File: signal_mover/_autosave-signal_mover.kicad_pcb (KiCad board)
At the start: 2 copper layers, 20.8 x 14.7 mm, 4 parts, among them P1 CONN_01X03

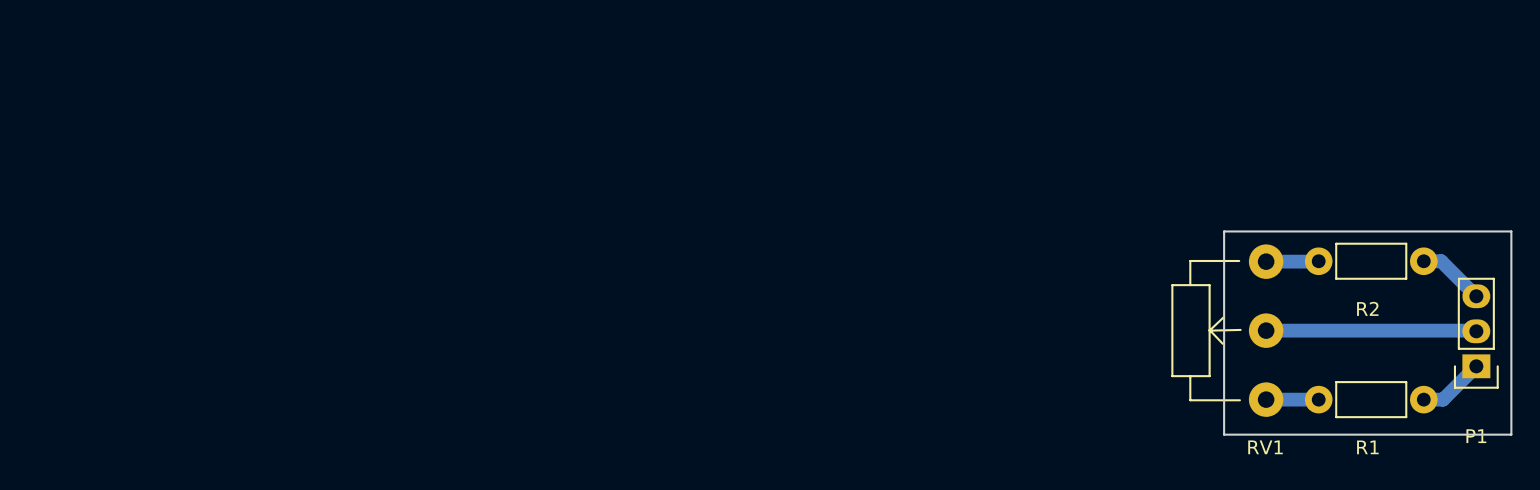
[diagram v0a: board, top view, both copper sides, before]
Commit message: updated signal mover
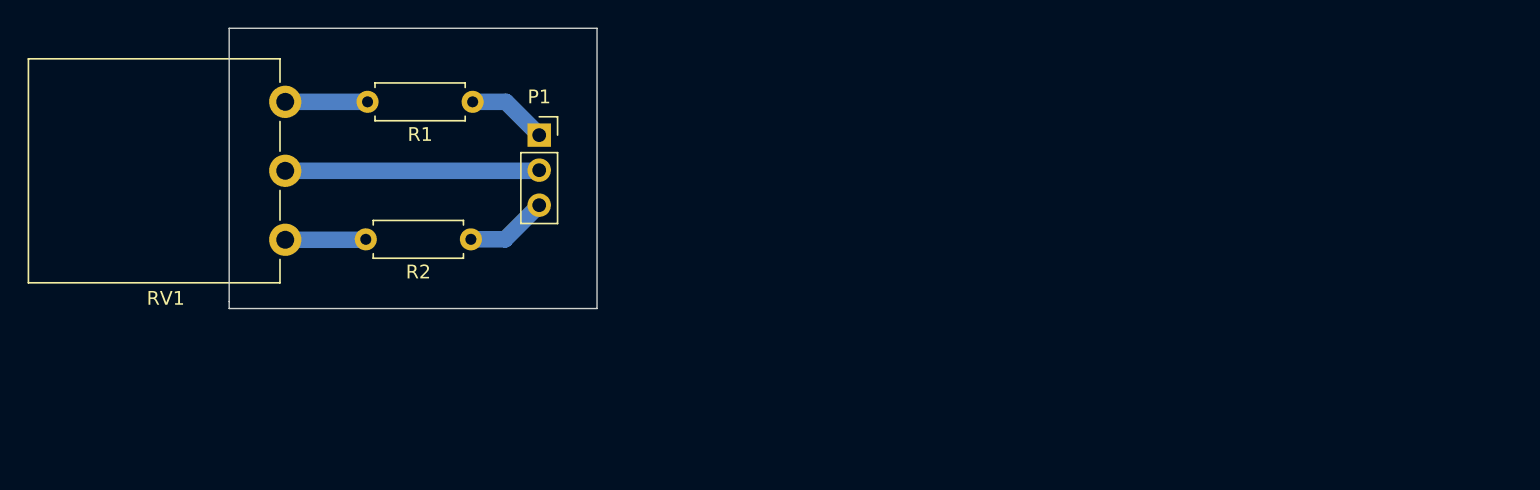
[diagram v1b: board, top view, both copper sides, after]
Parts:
- P1: footprint Pin_Headers:Pin_Header_Straight_1x03 -> Connector_PinSocket_2.54mm:PinSocket_1x03_P2.54mm_Vertical
- R1, R2: footprint Resistors_ThroughHole:Resistor_Horizontal_RM7mm -> Resistor_THT:R_Axial_DIN0207_L6.3mm_D2.5mm_P7.62mm_Horizontal
- RV1: footprint Potentiometers:Potentiometer_WirePads_largePads -> Potentiometer_THT:Potentiometer_Piher_PC-16_Single_Vertical
- moved RV1 74.3 mm to (67.6, 89.2)
- moved R1 72.3 mm to (81.2, 89.2)
- moved P1 70.0 mm to (86.0, 91.6), turned to 0 degrees
- moved R2 69.1 mm to (81.0, 99.1)
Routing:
- net Net-(P1-Pad2): track 15.3 -> 17.9 mm
- net Net-(R1-Pad2): track 3.81 -> 5.46 mm
- net Net-(R2-Pad2): track 3.82 -> 5.35 mm
- net Net-(P1-Pad3): track 4.86 -> 5.98 mm
- net Net-(P1-Pad1): track 4.81 -> 5.83 mm
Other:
- board size 20.8 x 14.7 mm -> 26.7 x 20.3 mm
- net class Default: clearance 0.3 -> 0.2; trace_width 1 -> 1.2; via_dia 0.6 -> 0.8
- rule pad_to_mask_clearance: 0.2 -> 0
- rule trace_clearance: 0.3 -> 0.2
